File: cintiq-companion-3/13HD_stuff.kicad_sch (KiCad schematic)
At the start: 22 parts, among them CN1 13HD_fingerpanel, J2 13HD_buttonboard, X1 13HD_eDP, X2 13HD_penpanel

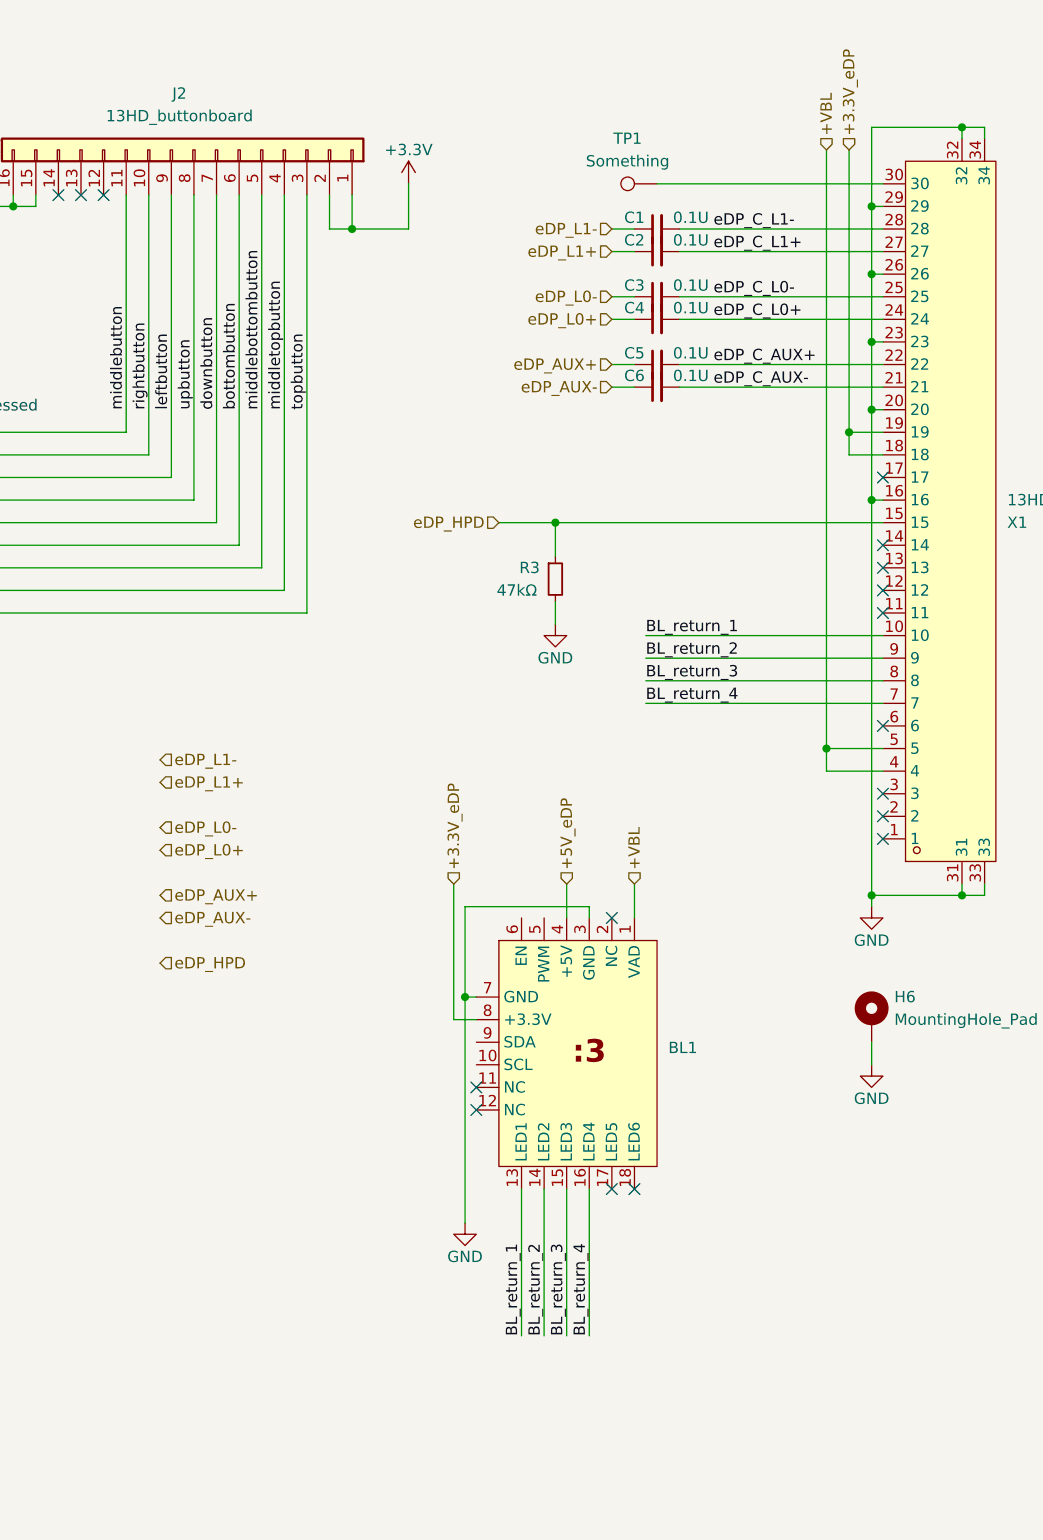
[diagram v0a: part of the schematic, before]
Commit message: Schematic in an ok state
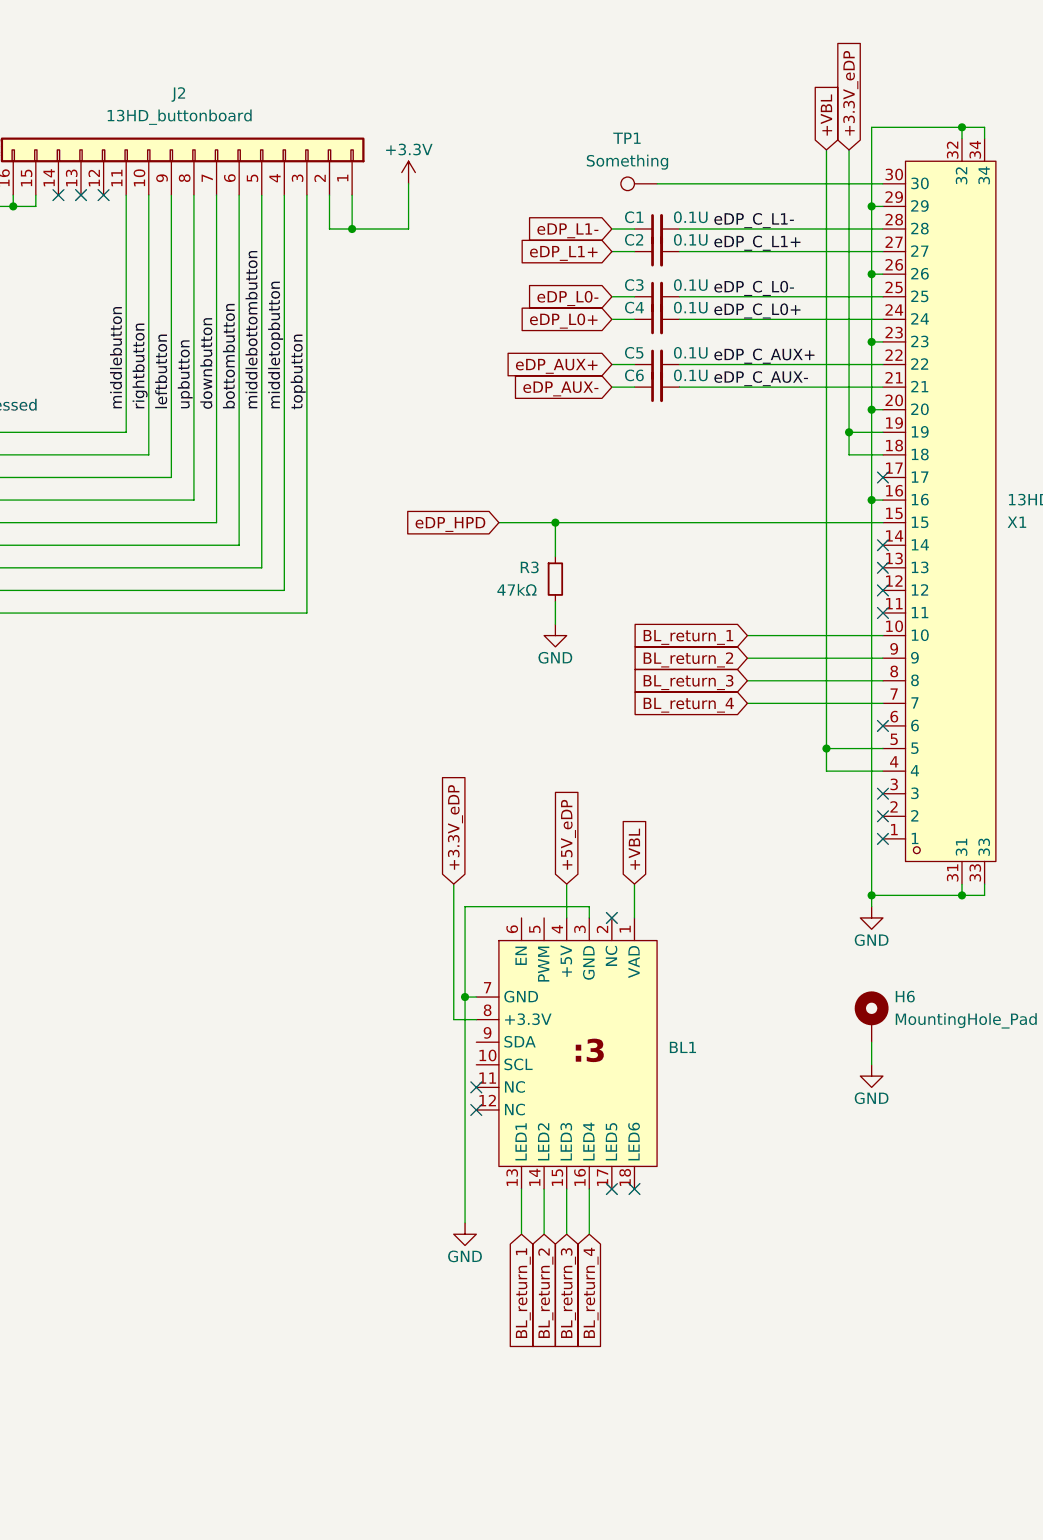
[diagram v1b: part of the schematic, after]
